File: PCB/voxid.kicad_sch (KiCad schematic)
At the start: 50 parts, among them J1 Conn_01x02_Pin, J2 Conn_01x02_Pin, J3 Conn_01x02_Pin, J4 v3.3, J5 v3.3, J6 AudioOut, J7 Conn_01x02_Pin, U1 TL072, U2 TL072, U3 TL072, U4 LM1117T-3.3

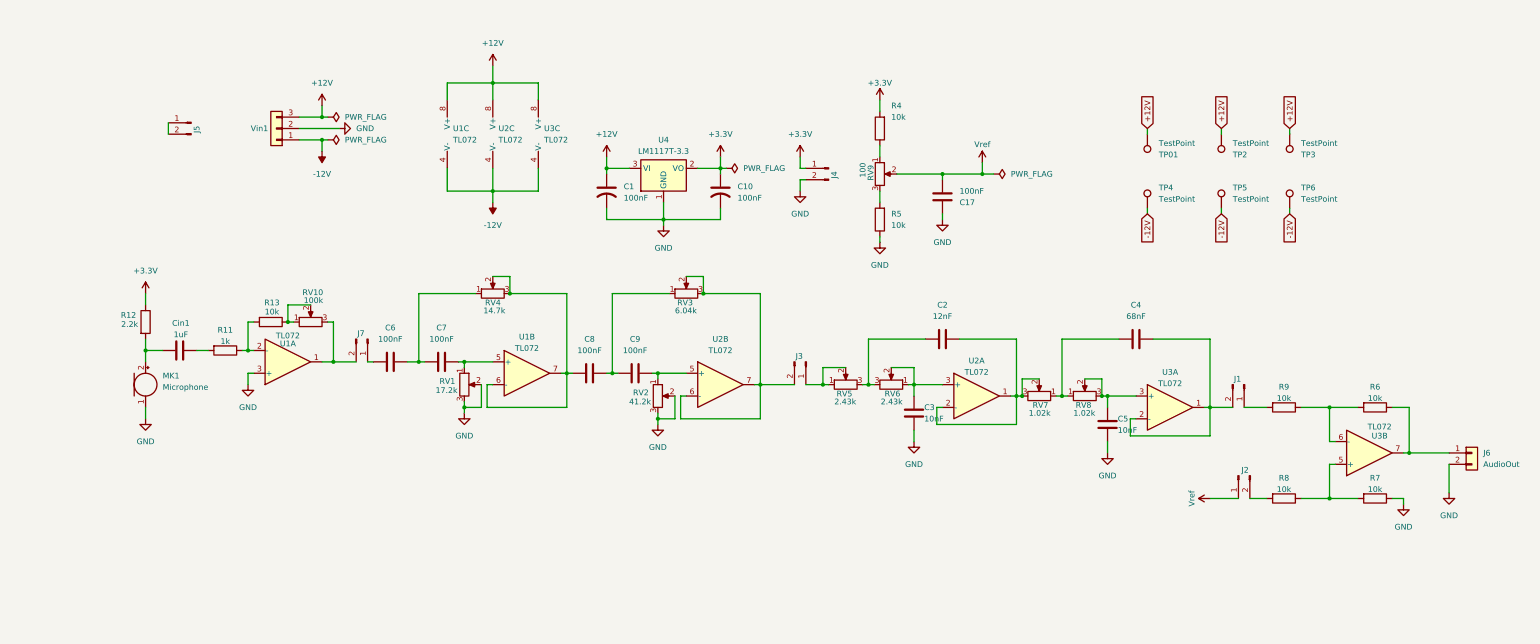
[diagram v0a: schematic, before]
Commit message: wip: Actualizacion de PCB y simulaciones
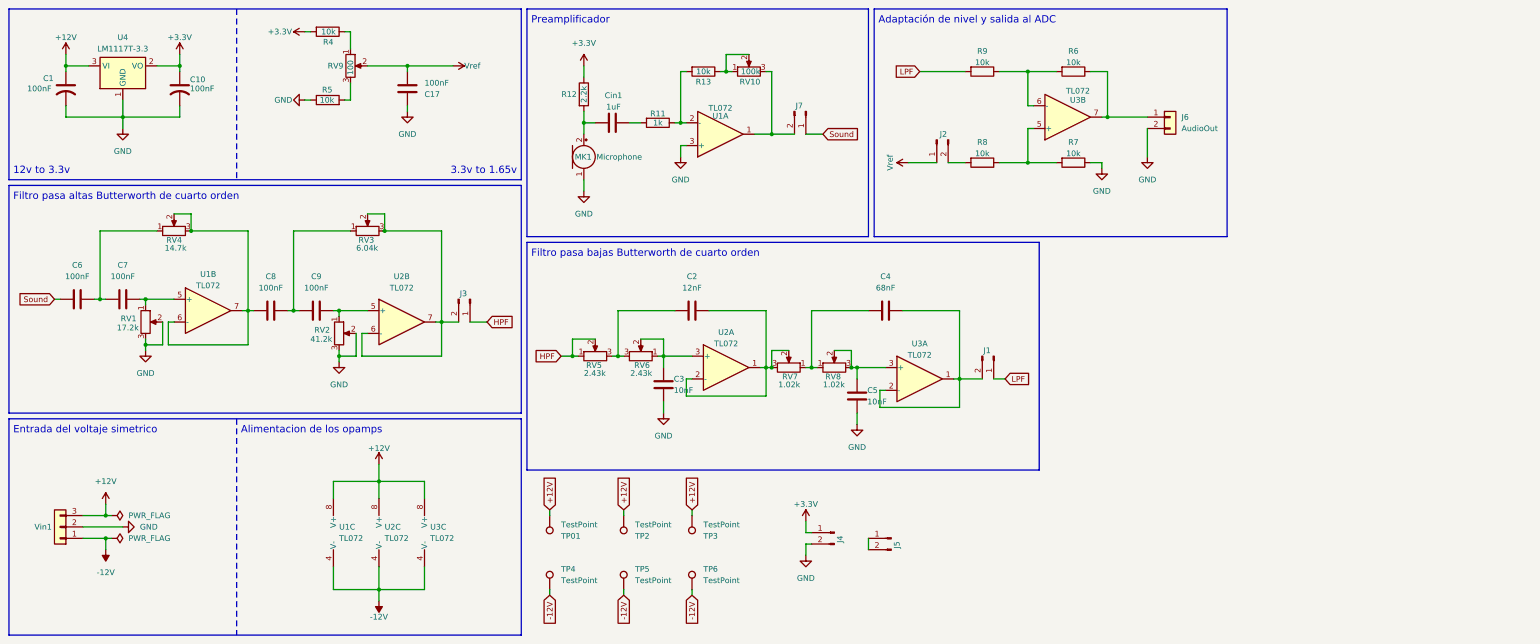
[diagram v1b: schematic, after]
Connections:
- net LPF: now reaches J1.1 (Pin_1), R9.2
- net Sound: now reaches C6.1, J7.1 (Pin_1)
- net HPF: now reaches J3.1 (Pin_1), RV5.1, RV5.2
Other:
- moved on the sheet: C1, C10, C17, C2, C3, C4, C5, C6, C7, C8, C9, Cin1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
